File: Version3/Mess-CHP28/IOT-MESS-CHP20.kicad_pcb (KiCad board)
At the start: 2 copper layers, 24.5 x 48.9 mm, 26 parts, among them J1 Jumper_2, J2 Jumper_2, J3 Jumper, J4 Conn_01x15_Pin, J5 Conn_01x15_Pin, J6 Jumper, J7 Jumper_2, J9 Jumper_2, K1 Crystal, U4 USB_C_Receptacle_USB2.0_16P, U5 ME6211C33M5, U6 XC6206PxxxMR

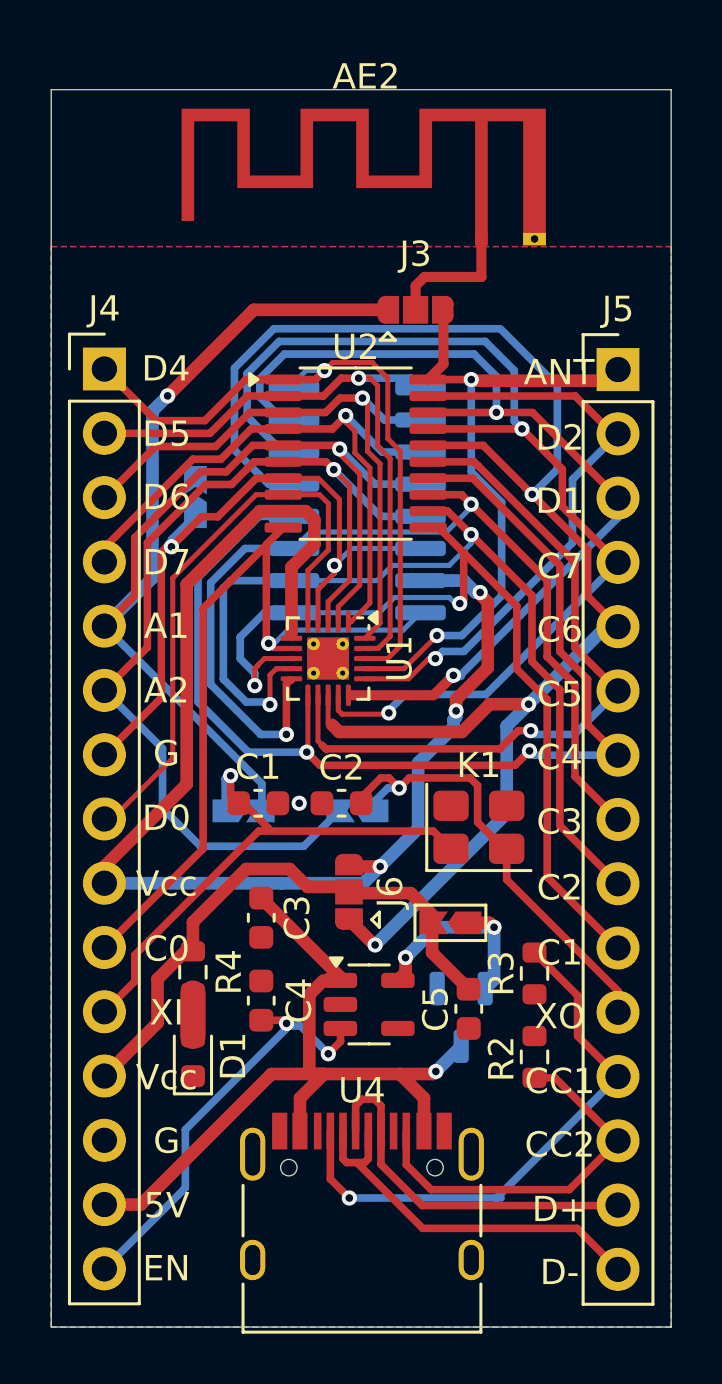
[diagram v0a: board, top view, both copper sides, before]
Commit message: update.
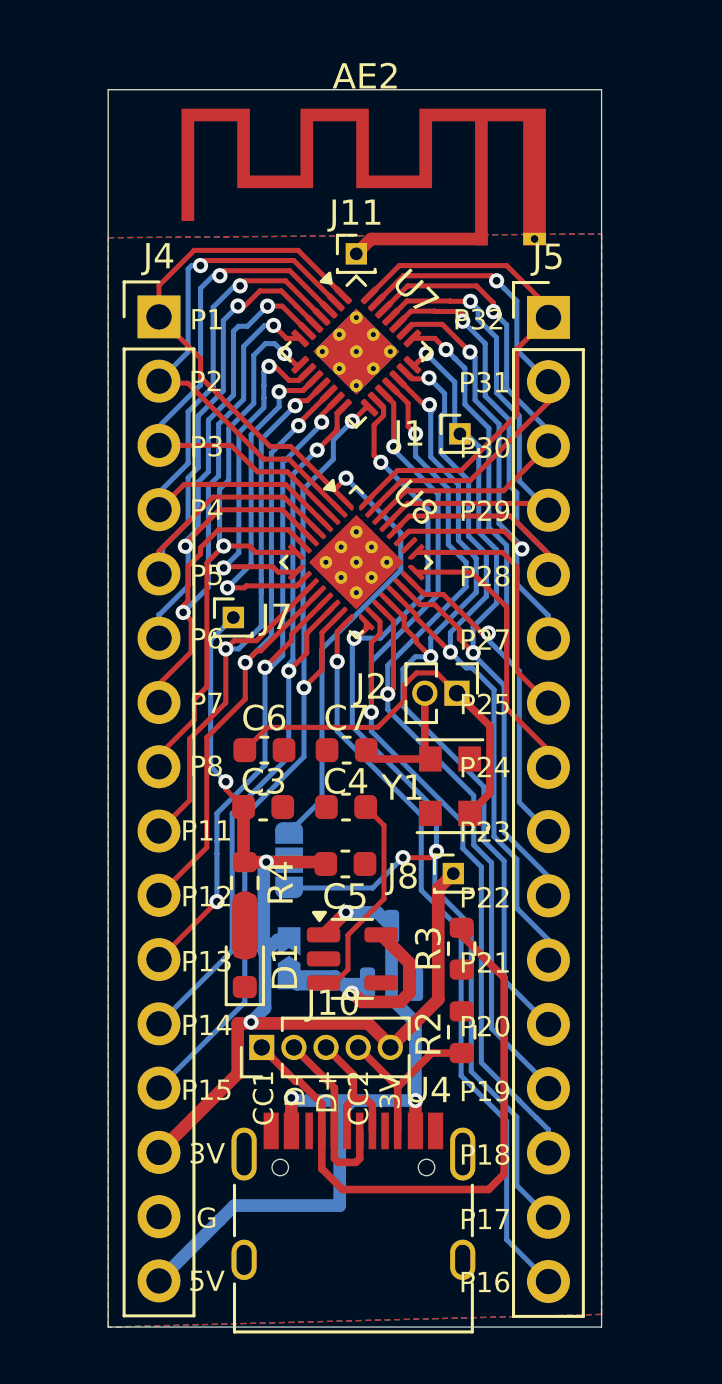
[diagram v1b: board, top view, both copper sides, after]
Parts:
- removed C1, C2: 12-25pF, Capacitor_SMD:C_0603_1608Metric
- removed J3: Jumper, IOT-Mess-Footprints:Jumper-3_P1.3mm_Open_RoundedPad1.0x1.5mm
- removed K1: Crystal, Crystal:Crystal_SMD_3225-4Pin_3.2x2.5mm
- removed U1: ~, Package_DFN_QFN:QFN-20-1EP_3x3mm_P0.4mm_EP1.65x1.65mm_ThermalVias
- removed U2: ~, Package_SO:TSSOP-20_4.4x6.5mm_P0.65mm
- removed U3: ~, Package_SO:SOP-16_3.9x9.9mm_P1.27mm
- added C6: 12-25pF, Capacitor_SMD:C_0603_1608Metric, F.Cu at (173.0, 113.0)
- added C7: 12-25pF, Capacitor_SMD:C_0603_1608Metric, F.Cu at (176.3, 113.0)
- added J10: Conn_01x05_Pin, Connector_PinHeader_1.27mm:PinHeader_1x05_P1.27mm_Vertical, F.Cu at (172.9, 124.8)
- added J11: Conn_01x01_Pin, Connector_PinHeader_1.00mm:PinHeader_1x01_P1.00mm_Vertical, F.Cu at (176.7, 93.4)
- added J8: Conn_01x01_Pin, Connector_PinHeader_1.00mm:PinHeader_1x01_P1.00mm_Vertical, F.Cu at (180.5, 117.9)
- added U7: ~, Package_DFN_QFN:QFN-28-1EP_4x4mm_P0.4mm_EP2.4x2.4mm_ThermalVias, F.Cu at (176.7, 97.2)
- added U8: ~, Package_DFN_QFN:QFN-32-1EP_4x4mm_P0.4mm_EP2.65x2.65mm_ThermalVias, F.Cu at (176.7, 105.6)
- added Y1: XO32, Oscillator:Oscillator_SMD_EuroQuartz_XO32-4Pin_3.2x2.5mm, F.Cu at (180.4, 114.4)
- J1, J7: value Jumper_2 -> Conn_01x01_Pin; footprint IOT-Mess-Footprints:Jumpper-triangle -> Connector_PinHeader_1.00mm:PinHeader_1x01_P1.00mm_Vertical; moved to F.Cu
- J2: value Jumper_2 -> Conn_01x02_Pin; footprint IOT-Mess-Footprints:Jumpper-triangle -> Connector_PinHeader_1.27mm:PinHeader_1x02_P1.27mm_Vertical; moved to F.Cu
- J4, J5: value Conn_01x15_Pin -> Conn_01x16_Pin; footprint Connector_PinHeader_2.54mm:PinHeader_1x15_P2.54mm_Vertical -> Connector_PinHeader_2.54mm:PinHeader_1x16_P2.54mm_Vertical
- J6, J9: moved to B.Cu
- moved G*** 17.3 mm to (176.8, 103.8)
- moved J1 17.2 mm to (180.8, 100.5)
- moved C4 8.35 mm to (176.2, 115.2), turned to 180 degrees
- moved C5 7.52 mm to (176.2, 117.5), turned to 0 degrees
- moved J9 6.53 mm to (174.0, 121.2), turned to 90 degrees
- moved J2 6.09 mm to (180.6, 110.8), turned to -90 degrees
- moved J7 4.99 mm to (171.8, 107.8), turned to 0 degrees
- moved C3 4.38 mm to (173.0, 115.2), turned to 0 degrees
- moved R4 4.08 mm to (172.2, 118.2)
- moved D1 4.08 mm to (172.2, 121.6)
- moved U6 3.68 mm to (178.1, 121.1), turned to 90 degrees
- moved J5 3.44 mm to (184.2, 95.9)
- moved R3 3.04 mm to (180.8, 120.8)
- moved R2 3.04 mm to (180.8, 124.1)
- moved J4 2.99 mm to (168.9, 95.9)
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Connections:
- AE2 pad 2: unconnected-(AE2-Shield-Pad2) -> GND
- C3 pad 1: 5V -> +3.3V
- C3 pad 2: P_0 -> GND
- C4 pad 2: P_0 -> GND
- C5 pad 2: P_0 -> GND
- D1 pad 1: P_0 -> GND
- J1 pad 1: OSCI -> P_22
- J2 pad 1: OSCO -> Net-(J2-Pin_1)
- J2 pad 2: P_6 -> Net-(J2-Pin_2)
- J4 pad 10: P_10 -> P_12
- J4 pad 11: OSCI -> P_13
- J4 pad 12: +3.3V -> P_14
- J4 pad 13: P_0 -> P_15
- J4 pad 14: 5V -> +3.3V
- J4 pad 15: LDO_EN -> GND
- J4 pad 9: P_9 -> P_11
- J5 pad 1: P_20 -> P_32
- J5 pad 10: P_11 -> P_22
- J5 pad 11: OSCO -> P_21
- J5 pad 12: CC1 -> P_20
- J5 pad 13: CC2 -> P_19
- J5 pad 14: D+ -> P_18
- J5 pad 15: D- -> P_17
- J5 pad 2: P_19 -> P_31
- J5 pad 3: P_18 -> P_30
- J5 pad 4: P_17 -> P_29
- J5 pad 5: P_16 -> P_28
- J5 pad 6: P_15 -> P_27
- J5 pad 7: P_14 -> P_25
- J5 pad 8: P_13 -> P_24
- J5 pad 9: P_12 -> P_23
- J6 pad 1: P_16 -> P_17
- J6 pad 3: P_9 -> P_1
- J7 pad 1: P_7 -> +3.3V
- R2 pad 2: P_0 -> GND
- R3 pad 2: P_0 -> GND
- U4 pad A1: P_0 -> GND
- U4 pad A12: P_0 -> GND
- U4 pad B1: P_0 -> GND
- U4 pad B12: P_0 -> GND
- U4 pad S1: P_0 -> GND
- U5 pad 2: P_0 -> GND
- U6 pad 1: P_0 -> GND
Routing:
- net P_9: track 52.5 -> 13.6 mm, vias 3 -> 2
- net P_16: track 65.3 -> 29.7 mm, vias 3 -> 1
- net P_5: track 55.1 -> 24.0 mm, vias 2 -> 1
- net P_21: track 0.00 -> 30.3 mm, vias 0 -> 2
- net P_22: track 0.00 -> 29.4 mm, vias 0 -> 2
- net P_23: track 0.00 -> 27.6 mm, vias 0 -> 2
- net P_28: track 0.00 -> 22.4 mm, vias 0 -> 1
- net OSCI: track 21.9 -> 0.00 mm, vias 1 -> 0
- net +3.3V: track 21.7 -> 42.9 mm, vias 0 -> 3
- net P_27: track 0.00 -> 21.1 mm, vias 0 -> 2
- net P_32: track 0.00 -> 20.4 mm
- net P_29: track 0.00 -> 19.7 mm, vias 0 -> 1
- net P_31: track 0.00 -> 19.6 mm, vias 0 -> 1
- net P_30: track 0.00 -> 18.7 mm, vias 0 -> 1
- net OSCO: track 18.6 -> 0.00 mm, vias 1 -> 0
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- added copper zone on B.Cu, net GND
- added copper zone on F.Cu, net GND
- removed copper zone on B.Cu, net P_0
- removed copper zone on F.Cu, net P_0
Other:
- board size 24.5 x 48.9 mm -> 19.5 x 48.9 mm
- board text added: "3V"
- board text added: "IOT_Mess P20 V3 1/30/26"
- board text added: "P1"
- board text added: "P11"
- board text added: "P12"
- board text added: "P13"
- board text added: "P14"
- board text added: "P15"
- board text added: "P16"
- board text added: "P17"
- board text added: "P18"
- board text added: "P19"
- board text added: "P2"
- board text added: "P20"
- board text added: "P21"
- board text added: "P22"
- board text added: "P23"
- board text added: "P24"
- board text added: "P25"
- board text added: "P27"
- board text added: "P28"
- board text added: "P29"
- board text added: "P3"
- board text added: "P30"
- board text added: "P31"
- board text added: "P32"
- board text added: "P4"
- board text added: "P5"
- board text added: "P6"
- board text added: "P7"
- board text added: "P8"
- board text removed: "A1"
- board text removed: "A2"
- board text removed: "ANT"
- board text removed: "C0"
- board text removed: "C1"
- board text removed: "C2"
- board text removed: "C3"
- board text removed: "C4"
- board text removed: "C5"
- board text removed: "C6"
- board text removed: "C7"
- board text removed: "D0"
- board text removed: "D1"
- board text removed: "D2"
- board text removed: "D4"
- board text removed: "D5"
- board text removed: "D6"
- board text removed: "D7"
- board text removed: "EN"
- board text removed: "IOT_Mess P20 V2.0 8/19/25"
- board text removed: "Vcc"
- board text removed: "XI"
- board text removed: "XO"
